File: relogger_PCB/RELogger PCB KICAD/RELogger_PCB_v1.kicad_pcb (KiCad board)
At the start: 2 copper layers, 73 parts, among them J1 RTC_MODULE, J2 Arduino_Nano_Header, J3 MICRO_SD, K1 ANEMOM1, P1 EXTERNAL PSU, P10 VANE, P11 SERIAL, P12 SOFT_SERIAL, P13 D6_D7, P14 AC_IN, P15 ANEMOM2, P2 BATTERY, P22 A_IN_45, P23 AGND_GND, P26 JMP_HALL, P3 SOLAR, P4 A_IN_01, P5 A_IN_23, P6 I2C_1, P7 I2C_2, P8 V_EXT, P9 3V3_VREF, Q2 RFU9110PBF, SW1 CALIBRATE, SW2 SW_PUSH_SMALL_H, SW3 ON/OFF, SW4 SW_PUSH_SMALL_H, U1 MCP3208, U2 MCP1826S, U3 LM2574, U5 MCP73832, U6 LM393

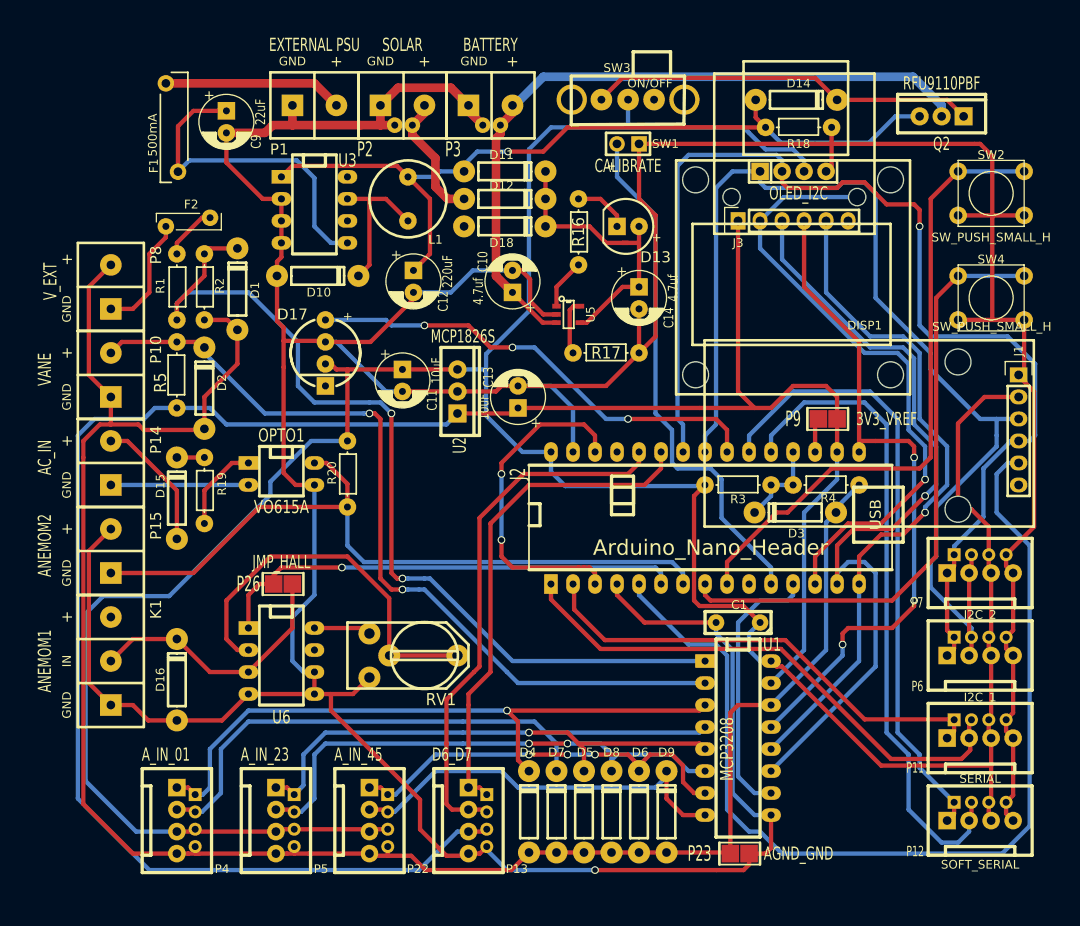
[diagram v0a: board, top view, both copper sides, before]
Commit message: Small PCB updates
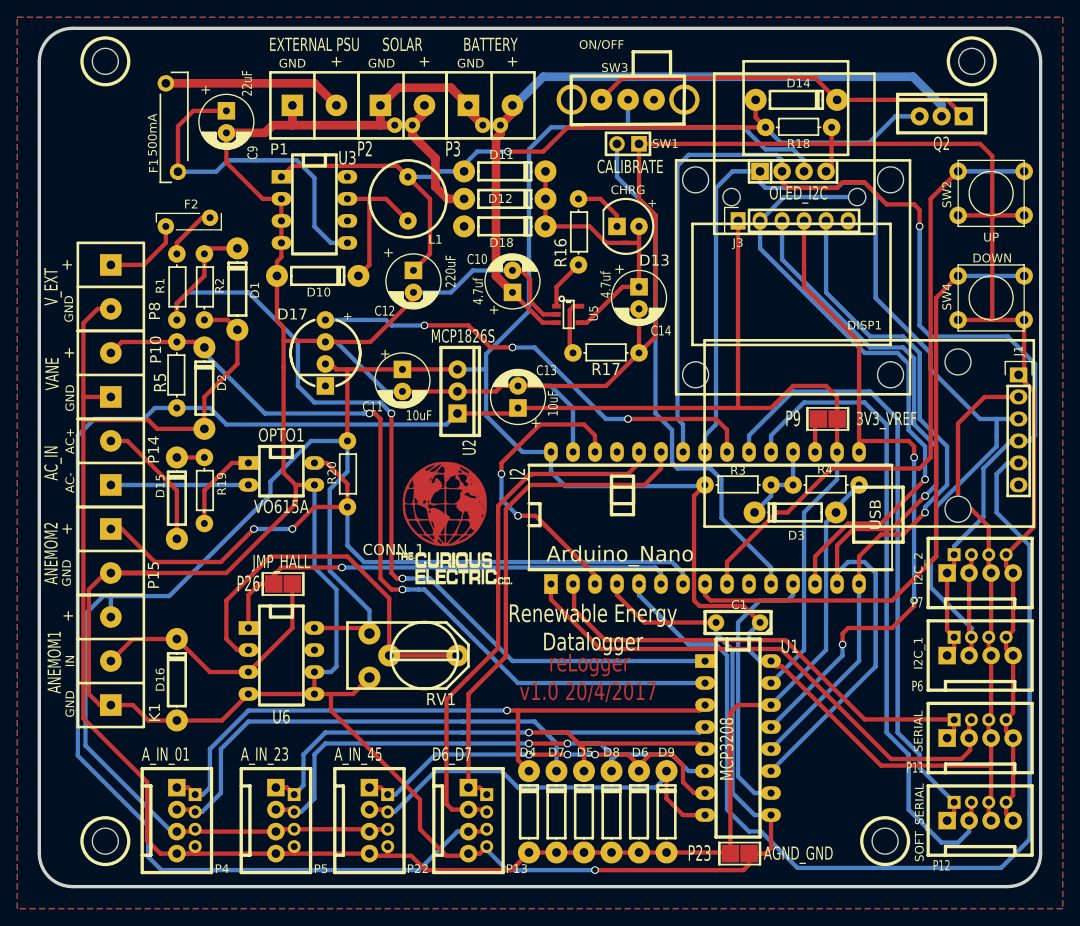
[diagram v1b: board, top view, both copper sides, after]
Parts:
- added HOLE1: CONN_1, 3mm_hole_relogger, F.Cu at (85.1, 36.8)
- added LOGO1: CONN_1, CuriousElectric3:CEC_Globe_10mm_FCU, F.Cu at (124.3, 87.9)
- added LOGO2: CONN_1, CuriousElectric3:TCEC_Words_13mm, F.Cu at (118.4, 93.2)
- J2: value Arduino_Nano_Header -> Arduino_Nano
- SW2: value SW_PUSH_SMALL_H -> UP
- SW4: value SW_PUSH_SMALL_H -> DOWN
- moved P15 5.08 mm to (85.7, 90.8), turned to 270 degrees
- moved P8 5.08 mm to (85.7, 60.3), turned to 270 degrees
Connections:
- K1 pad 3: (no net) -> /Vss
- RV1 pad 1: /Hall_to_freq/Vss -> /Vss
- U6 pad 8: /Hall_to_freq/Vss -> /Vss
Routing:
- net /Vss: track 342.5 -> 376.6 mm
- net GND: track 544.3 -> 576.4 mm
- net /Hall_to_freq/Vss: track 6.61 -> 0.00 mm
- net Net-(F2-Pad1): track 13.6 -> 9.31 mm
- net /Arduino Uno/RESET: track 38.7 -> 34.7 mm
- net /CLK_INT: track 115.7 -> 118.0 mm
- net GNDA: track 227.9 -> 225.9 mm
- net +3.3V: track 245.1 -> 243.6 mm
- net /IN_ACFREQ: track 83.7 -> 84.8 mm, vias 0 -> 2
- net /A0: track 76.7 -> 76.2 mm
- added copper zone on B.Cu, net GND
- added copper zone on F.Cu, net GND
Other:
- board outline added: 115.6 x 99.1 mm
- board text added: "Renewable Energy Datalogger"
- board text added: "reLogger"
- board text added: "v1.0 20/4/2017"

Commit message: BOM uploaded
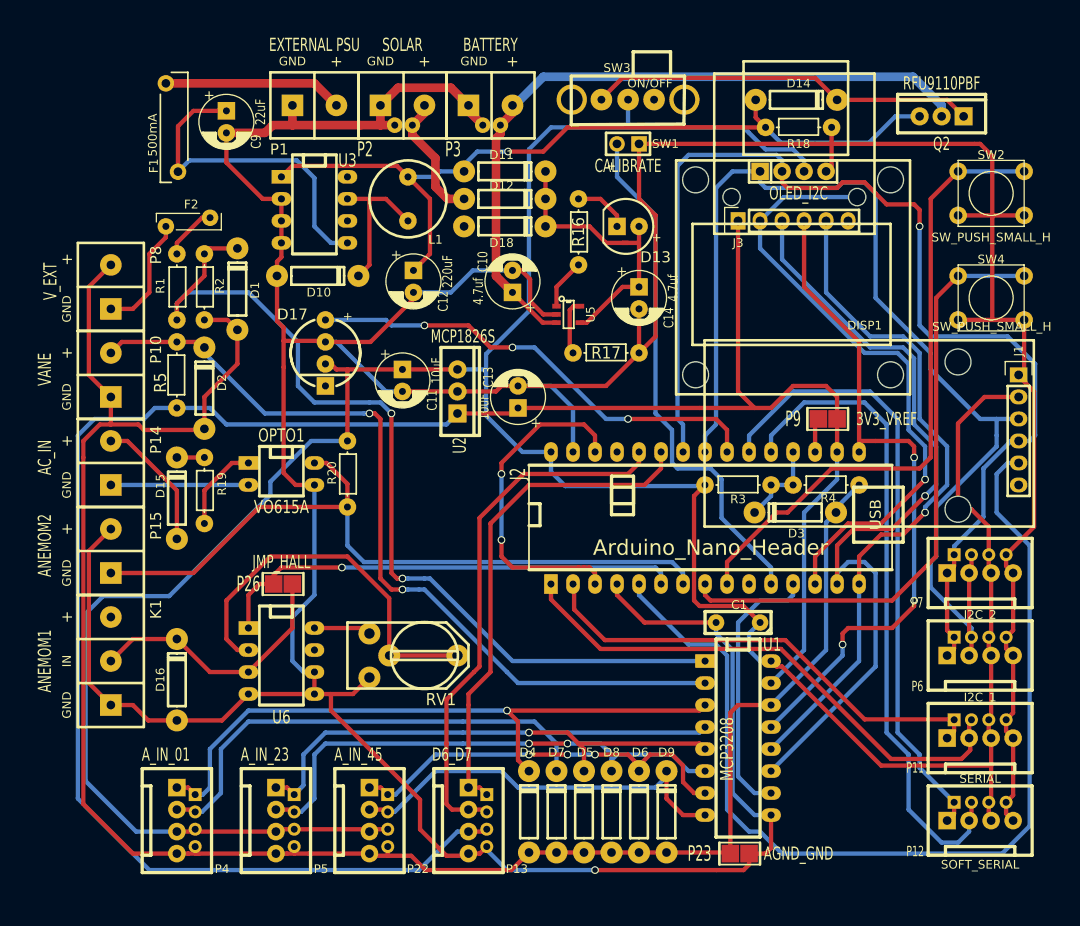
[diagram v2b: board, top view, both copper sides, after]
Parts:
- removed HOLE1: CONN_1, 3mm_hole_relogger
- removed LOGO1: CONN_1, CuriousElectric3:CEC_Globe_10mm_FCU
- removed LOGO2: CONN_1, CuriousElectric3:TCEC_Words_13mm
- J2: value Arduino_Nano -> Arduino_Nano_Header
- SW2: value UP -> SW_PUSH_SMALL_H
- SW4: value DOWN -> SW_PUSH_SMALL_H
- moved P15 5.08 mm to (85.7, 95.9), turned to 90 degrees
- moved P8 5.08 mm to (85.7, 65.4), turned to 90 degrees
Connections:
- K1 pad 3: /Vss -> (no net)
- RV1 pad 1: /Vss -> /Hall_to_freq/Vss
- U6 pad 8: /Vss -> /Hall_to_freq/Vss
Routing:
- net /Vss: track 376.6 -> 342.5 mm
- net GND: track 576.4 -> 544.3 mm
- net /Hall_to_freq/Vss: track 0.00 -> 6.61 mm
- net Net-(F2-Pad1): track 9.31 -> 13.6 mm
- net /Arduino Uno/RESET: track 34.7 -> 38.7 mm
- net /CLK_INT: track 118.0 -> 115.7 mm
- net GNDA: track 225.9 -> 227.9 mm
- net +3.3V: track 243.6 -> 245.1 mm
- net /IN_ACFREQ: track 84.8 -> 83.7 mm, vias 2 -> 0
- net /A0: track 76.2 -> 76.7 mm
- removed copper zone on B.Cu, net GND
- removed copper zone on F.Cu, net GND
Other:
- board outline removed
- board text removed: "Renewable Energy Datalogger"
- board text removed: "reLogger"
- board text removed: "v1.0 20/4/2017"
